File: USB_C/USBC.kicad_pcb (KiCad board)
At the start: 2 copper layers, 20.6 x 16.3 mm, 9 parts, among them J1 USB_C_Receptacle_USB2.0, J2 Conn_01x08

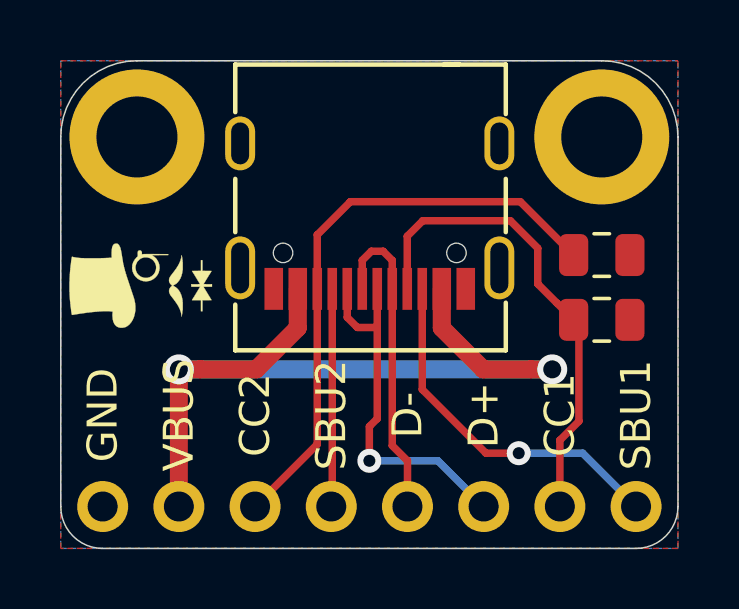
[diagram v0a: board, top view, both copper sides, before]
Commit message: Board Redesign
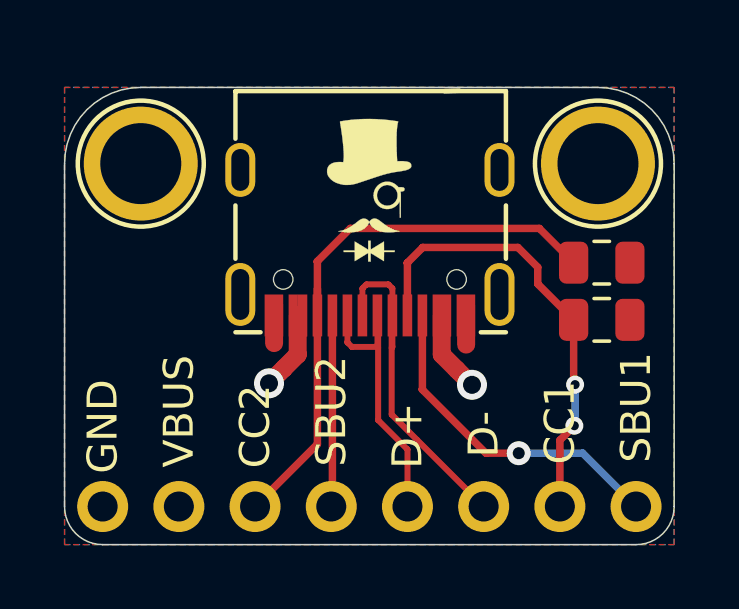
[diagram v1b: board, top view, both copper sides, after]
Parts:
- G***: footprint logo:logo94x134 -> logo:logo76x107
- H1, H2: footprint MountingHole:MountingHole_2.7mm_M2.5_ISO14580_Pad -> SirBoardLibrary:MountingHole_M2.5_SirBoard
- J1: footprint U_FL:USB_C -> SirBoardLibrary:USB_C
- moved H2 15.4 mm to (58.0, 31.5)
- moved H1 15.4 mm to (73.3, 31.5)
- moved G*** 8.26 mm to (65.7, 32.4), turned to 0 degrees
- moved J1 1.58 mm to (68.9, 37.1)
- moved R2 0.25 mm to (73.4, 34.8)
- moved G*** 0.13 mm to (65.7, 39.9)
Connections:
- J2 pad 4: /SBU2 -> /SBU1
- J2 pad 5: /D- -> /D+
- J2 pad 6: /D+ -> /D-
- J2 pad 8: /SBU1 -> /SBU2
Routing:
- net /VBUS: track 28.4 -> 5.38 mm
- net /SBU1: track 12.1 -> 6.43 mm, vias 1 -> 0
- net /SBU2: track 7.27 -> 11.2 mm, vias 0 -> 1
- net GND: track 0.00 -> 3.67 mm
- net /D+: track 12.4 -> 9.64 mm, vias 1 -> 0
- net /CC1: track 16.1 -> 15.3 mm, vias 0 -> 2
- net /D-: track 10.6 -> 11.5 mm
- added copper zone on B.Cu, net /VBUS
- removed copper zone on B.Cu, net GND
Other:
- board size 20.6 x 16.3 mm -> 20.3 x 15.2 mm
